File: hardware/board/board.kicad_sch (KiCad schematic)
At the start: 8 parts, among them J101 UART, J102 CM4_DEBUG, J103 DEBUG_PORT, U101 Oled

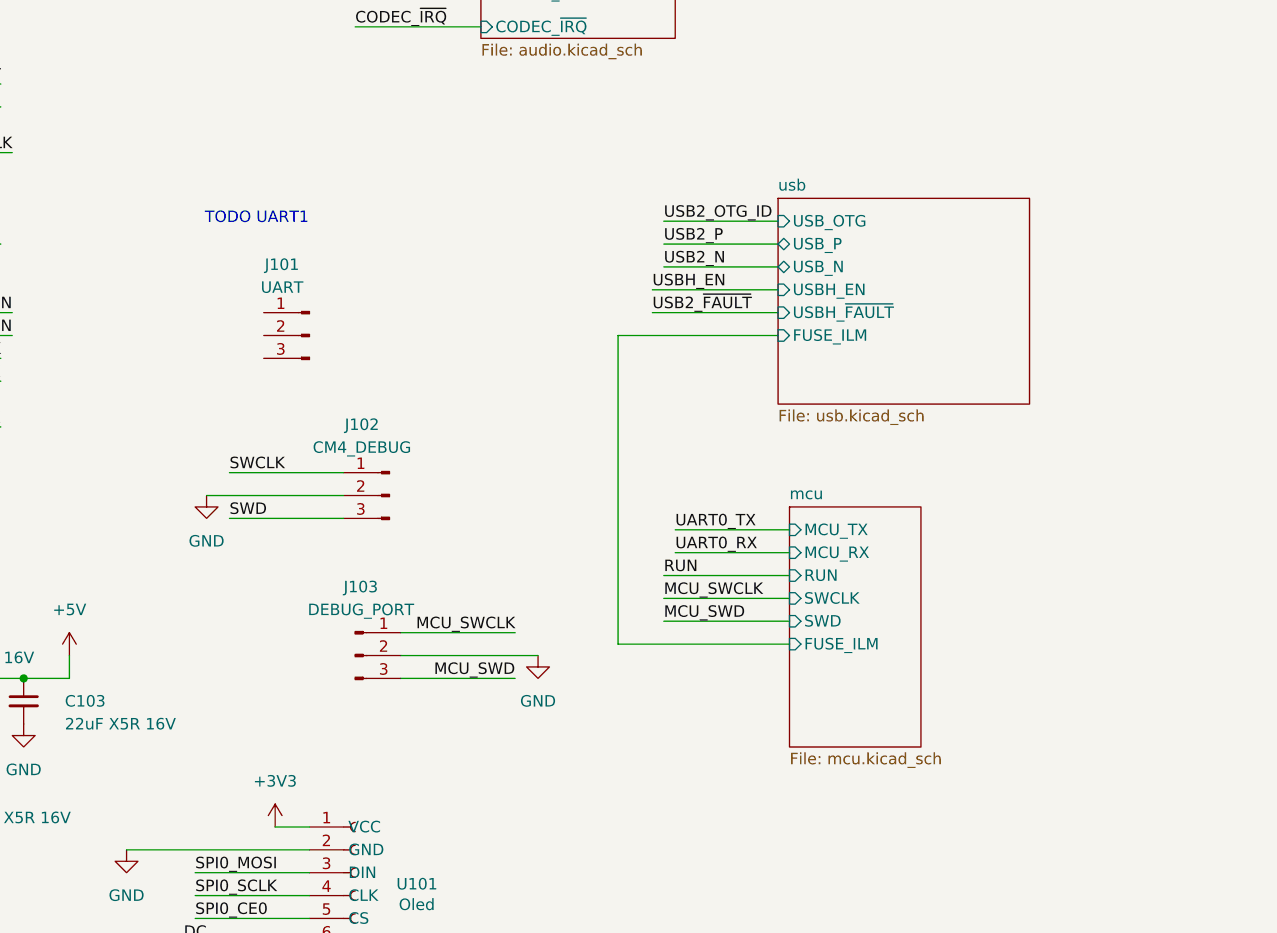
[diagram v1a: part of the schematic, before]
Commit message: loose ends
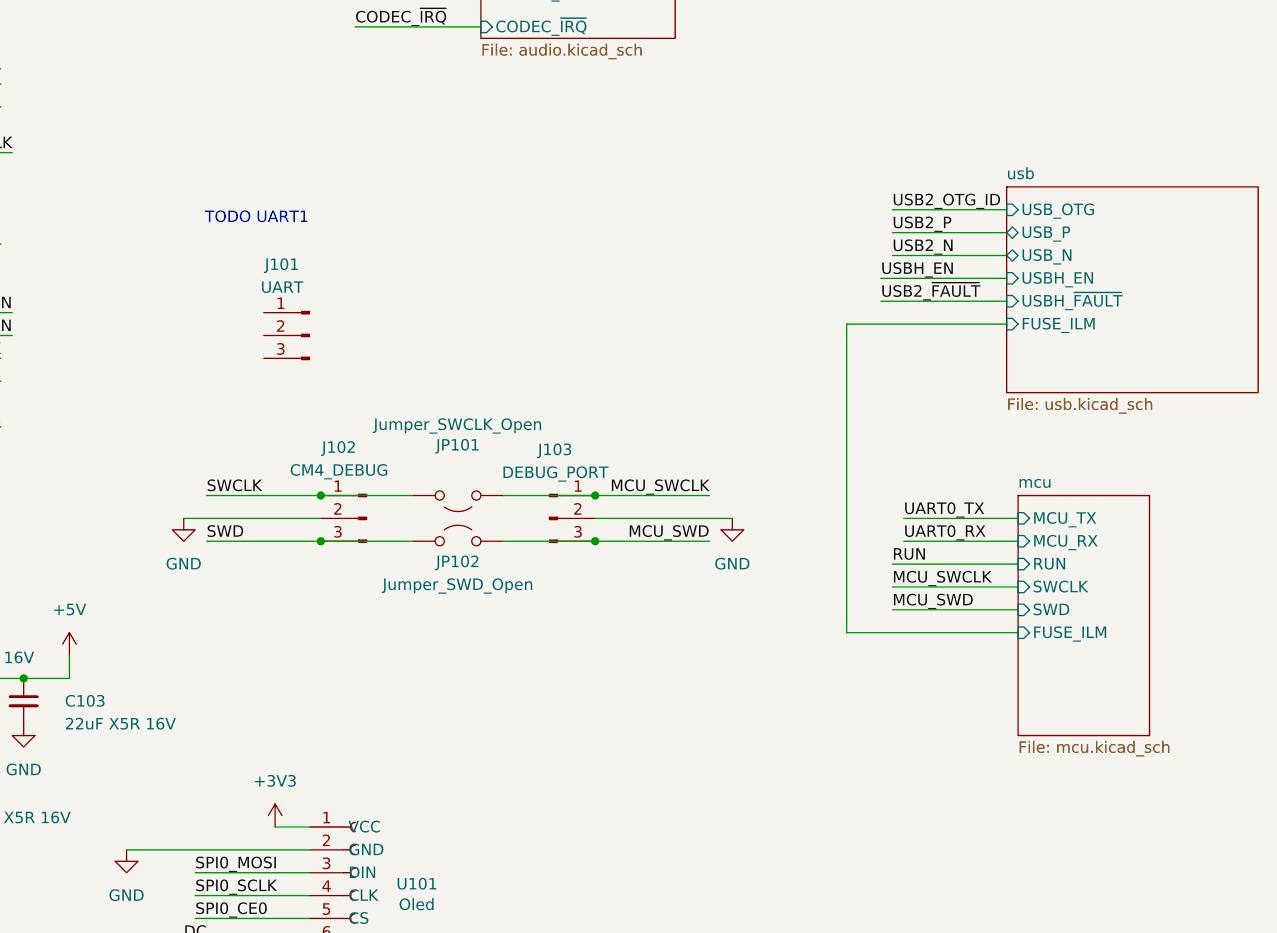
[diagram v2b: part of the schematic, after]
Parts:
- added JP101: Jumper_SWCLK_Open, Jumper:SolderJumper-2_P1.3mm_Open_TrianglePad1.0x1.5mm, symbol Jumper:Jumper_2_Open
- added JP102: Jumper_SWD_Open, Jumper:SolderJumper-2_P1.3mm_Open_TrianglePad1.0x1.5mm, symbol Jumper:Jumper_2_Open
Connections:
- net MCU_SWCLK: now also JP101.1 (A)
- net MCU_SWD: now also JP102.1 (A)
- net SWCLK: now also JP101.2 (B)
- net SWD: now also JP102.2 (B)
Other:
- moved on the sheet: J102, J103

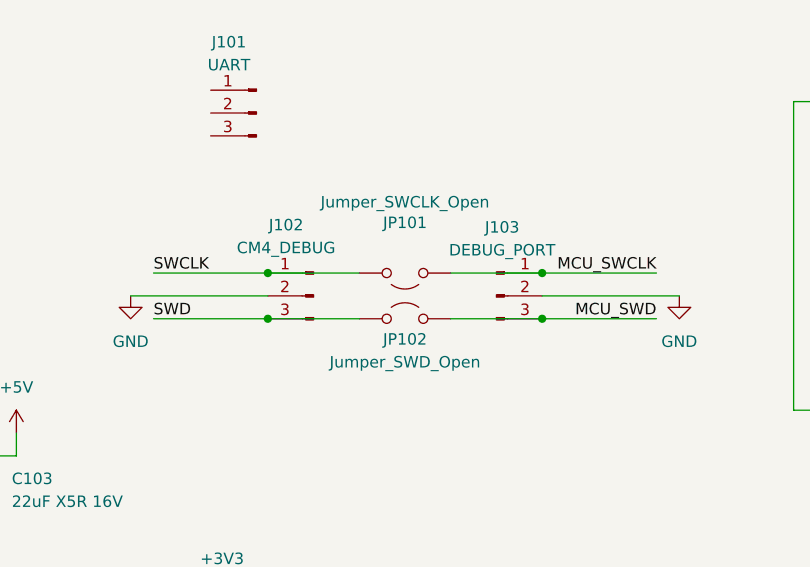
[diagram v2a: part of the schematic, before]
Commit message: swd swclk run
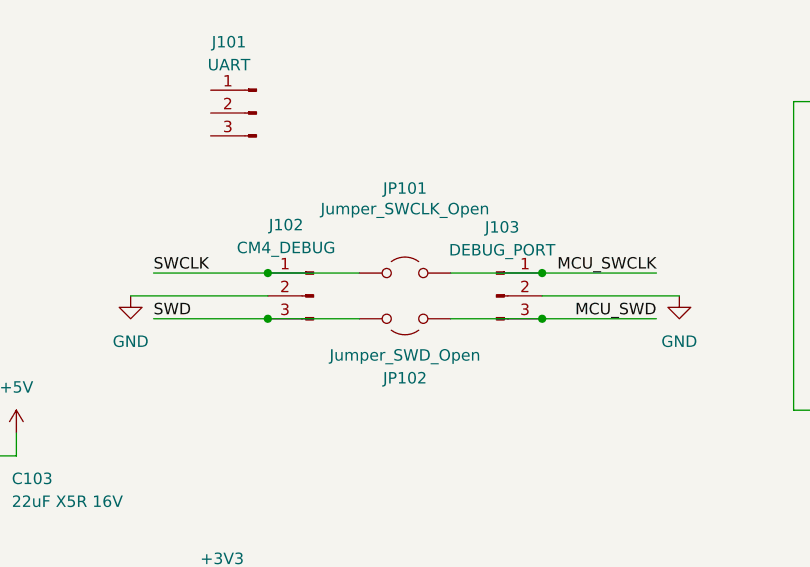
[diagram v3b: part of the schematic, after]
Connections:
- net MCU_SWCLK: now also JP101.2 (B); no longer JP101.1 (A)
- net MCU_SWD: now also JP102.2 (B); no longer JP102.1 (A)
- net SWCLK: now also JP101.1 (A); no longer JP101.2 (B)
- net SWD: now also JP102.1 (A); no longer JP102.2 (B)
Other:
- moved on the sheet: JP101, JP102
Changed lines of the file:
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@@
 		(lib_id "Jumper:Jumper_2_Open")
 		(at 276.86 128.27 0)
-		(mirror y)
+		(mirror x)
 		(unit 1)
 		(body_style 1)
@@
 		(dnp no)
 		(property "Reference" "JP102"
-			(at 276.86 130.556 0)
+			(at 276.86 134.874 0)
 			(show_name no)
 			(do_not_autoplace no)
@@
 		)
 		(property "Value" "Jumper_SWD_Open"
-			(at 276.86 133.096 0)
+			(at 276.86 132.334 0)
 			(show_name no)
 			(do_not_autoplace no)
@@
 	(symbol
 		(lib_id "Jumper:Jumper_2_Open")
-		(at 276.86 123.19 180)
+		(at 276.86 123.19 0)
 		(unit 1)
 		(body_style 1)
@@
 		(dnp no)
 		(property "Reference" "JP101"
-			(at 276.86 117.602 0)
+			(at 276.86 113.792 0)
 			(show_name no)
 			(do_not_autoplace no)
@@
 		)
 		(property "Value" "Jumper_SWCLK_Open"
-			(at 276.86 115.316 0)
-			(show_name no)
-			(do_not_autoplace no)
+			(at 276.86 116.078 0)
+			(show_name no)
+			(do_not_autoplace no)
